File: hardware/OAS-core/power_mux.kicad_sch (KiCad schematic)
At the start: 2 parts, among them U2 LM66200, U9 LM66100DCK

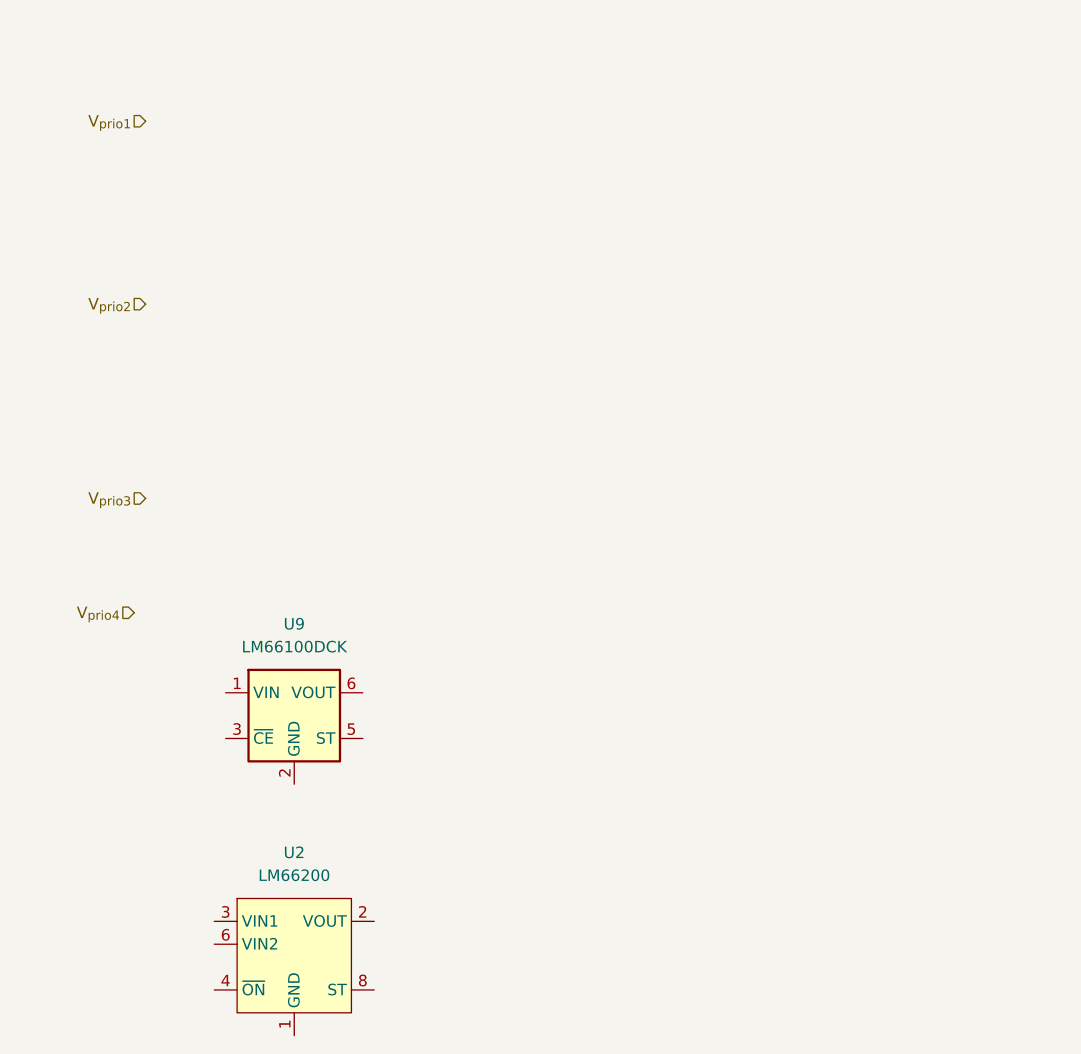
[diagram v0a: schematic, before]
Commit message: Mux
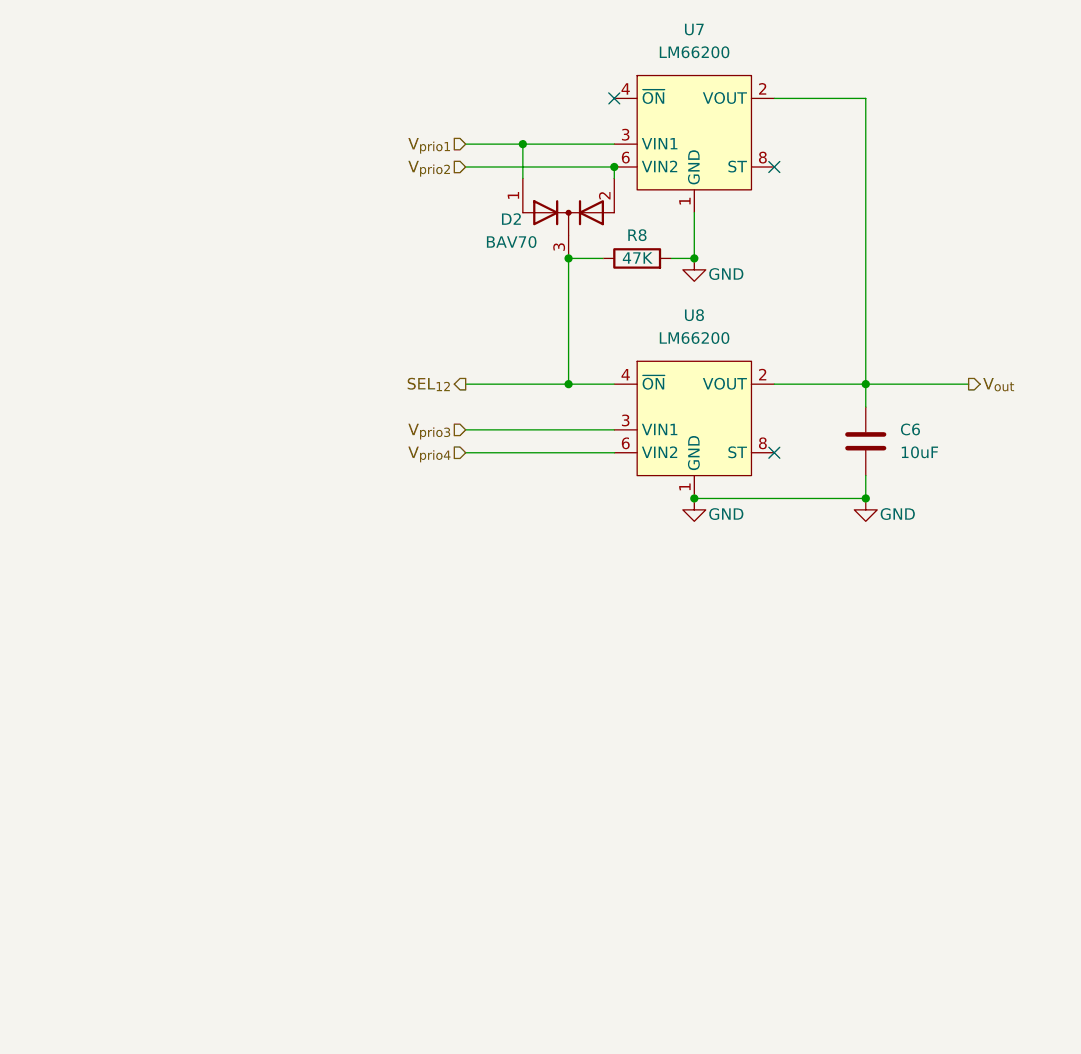
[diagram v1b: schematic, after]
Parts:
- removed U2: LM66200, Package_SON:Texas_R-PUSON-N8_USON-8-1EP_1.6x2.1mm_P0.5mm_EP0.4x1.7mm, symbol oas:LM66200
- removed U9: LM66100DCK, Package_TO_SOT_SMD:SOT-363_SC-70-6, symbol Power_Management:LM66100DCK
- added C6: 10uF, symbol Device:C
- added D2: BAV70, Package_TO_SOT_SMD:SOT-23, symbol Diode:BAV70
- added R8: 47K, symbol Device:R
- added U7, U8: LM66200, Package_SON:Texas_R-PUSON-N8_USON-8-1EP_1.6x2.1mm_P0.5mm_EP0.4x1.7mm, symbol oas:LM66200
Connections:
- net V_{prio1}: now also D2.1 (A), U7.3 (VIN1)
- net V_{prio2}: now also D2.2 (A), U7.6 (VIN2)
- net V_{prio3}: now also U8.3 (VIN1)
- net V_{prio4}: now also U8.6 (VIN2)
- new net GND: C6.2, R8.2, U7.1 (GND), U7.5 (GND), U8.1 (GND), U8.5 (GND)
- new net SEL_{12}: D2.3 (K), R8.1, U8.4 (~{ON})
- new net V_{out}: C6.1, U7.2 (VOUT), U7.7 (VOUT), U8.2 (VOUT), U8.7 (VOUT)
- no-connect marks 0 -> 3
